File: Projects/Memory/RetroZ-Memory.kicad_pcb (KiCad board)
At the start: 2 copper layers, 100 x 80 mm, 17 parts, among them J1 Client Bus, U1 74LS32, U2 AT28C64B-15PU, U3 74LS138, U5 74LS08, U6 AS6C4008-55PCN, U7 74HC273, U8 74LS08-And2

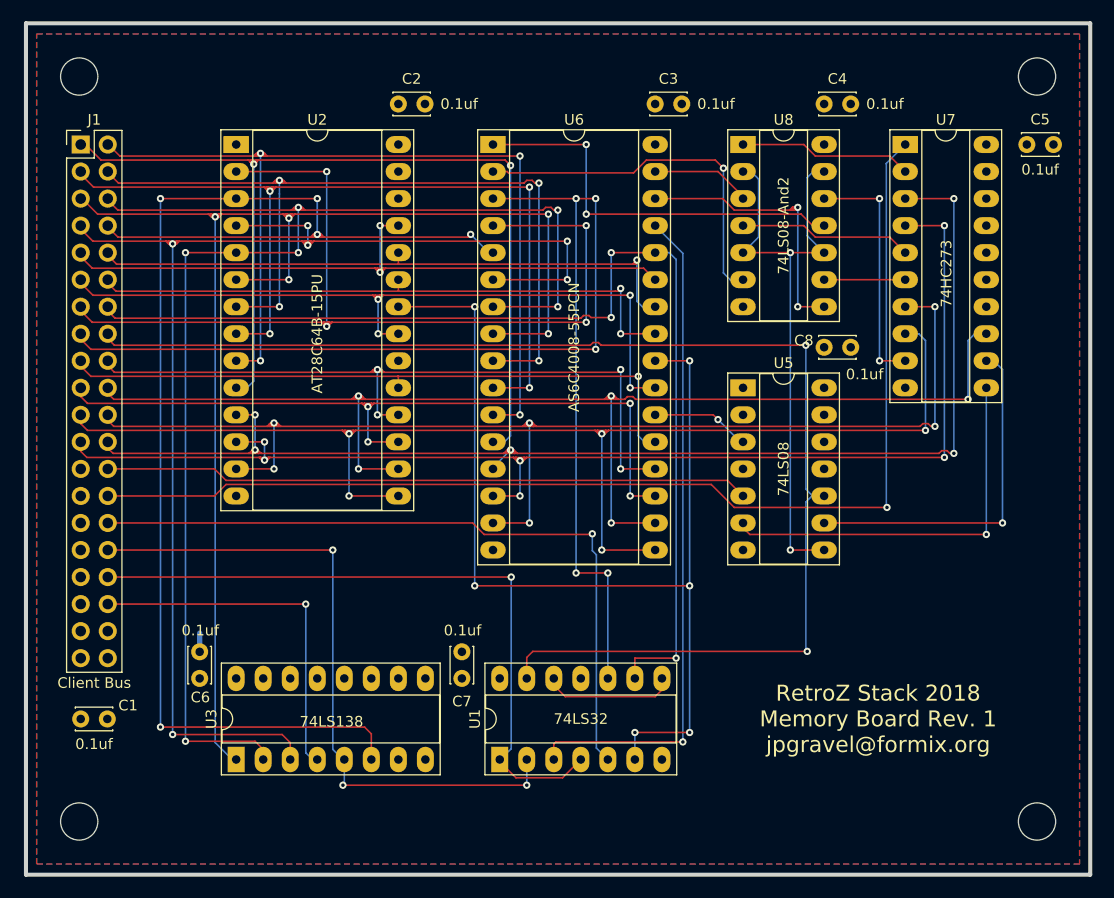
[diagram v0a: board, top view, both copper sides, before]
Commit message: sio2+ctc
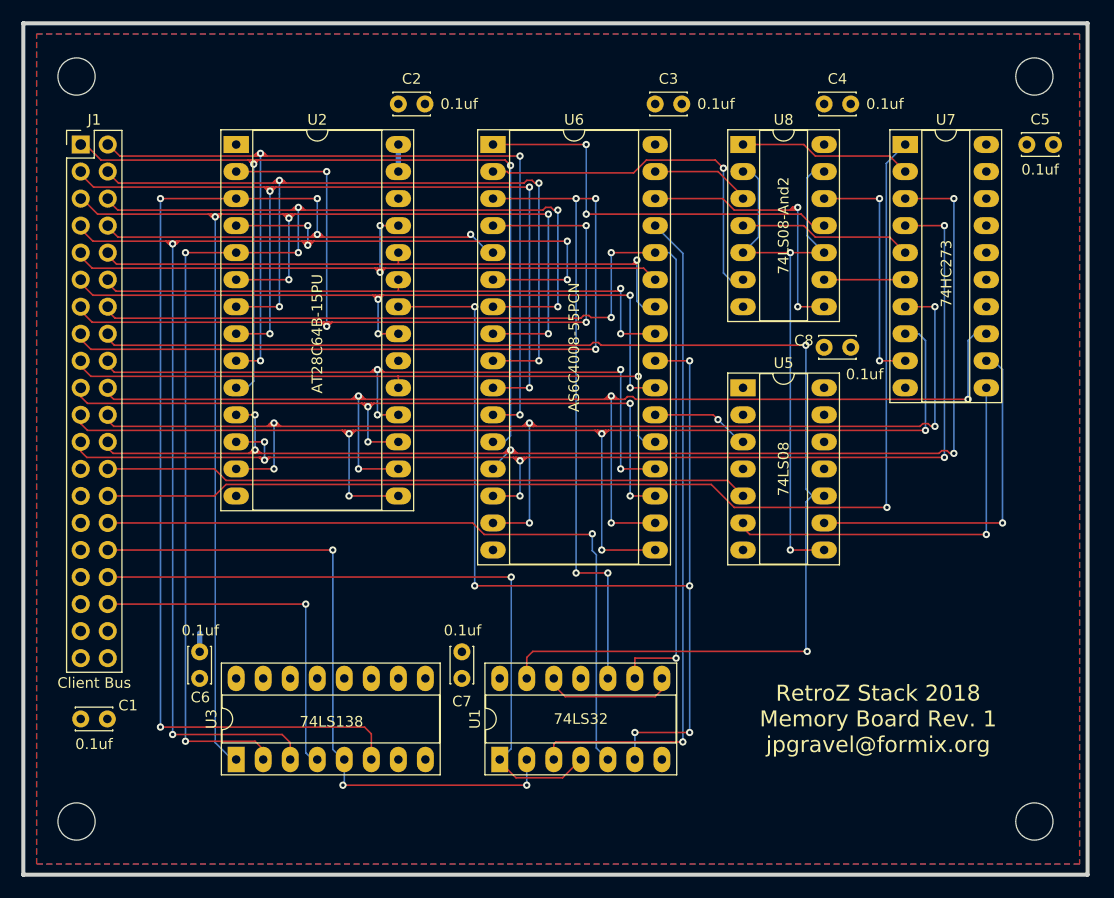
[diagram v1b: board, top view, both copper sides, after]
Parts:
- moved REF** 0.25 mm to (107.0, 141.0)
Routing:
- net VCC: track 0.00 -> 2.54 mm
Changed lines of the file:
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@@
   (general
     (links 118)
-    (no_connects 2)
+    (no_connects 1)
     (area 106.8476 53.7126 207.592701 149.6474)
     (thickness 1.6)
     (drawings 1)
-    (tracks 903)
+    (tracks 904)
     (zones 0)
     (modules 17)
@@
   )
   (module EuroBoard_Outline:EuroBoard_halb_Type-I_100mmX80mm_holes (layer F.Cu)
-    (at 107.25 141)
+    (at 107 141)
     (descr "Outline, Eurocard 1/2, Type I, 100x80mm, with holes 3,5mm")
     (tags "Outline, Eurocard 1/2, Type I, 100x80mm, with holes 3,5mm")
@@
     (effects (font (size 1.5 1.5) (thickness 0.3)))
   )
+  (segment (start 142.24 74.93) (end 142.24 72.39) (width 0.5) (layer B.Cu) (net 1) (status C00000))
   (segment (start 123.571 120.055) (end 123.571 118.3005) (width 0.5) (layer B.Cu) (net 2))
   (segment (start 128.397 73.8505) (end 128.397 73.9775) (width 0.1524) (layer F.Cu) (net 3))
